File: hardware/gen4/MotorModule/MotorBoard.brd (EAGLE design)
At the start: 32.6 x 58.8 mm, 65 parts, among them IC1 XMEGA16A4A, M1O1 TEST_PT, M1O2 TEST_PT, M1O3 TEST_PT

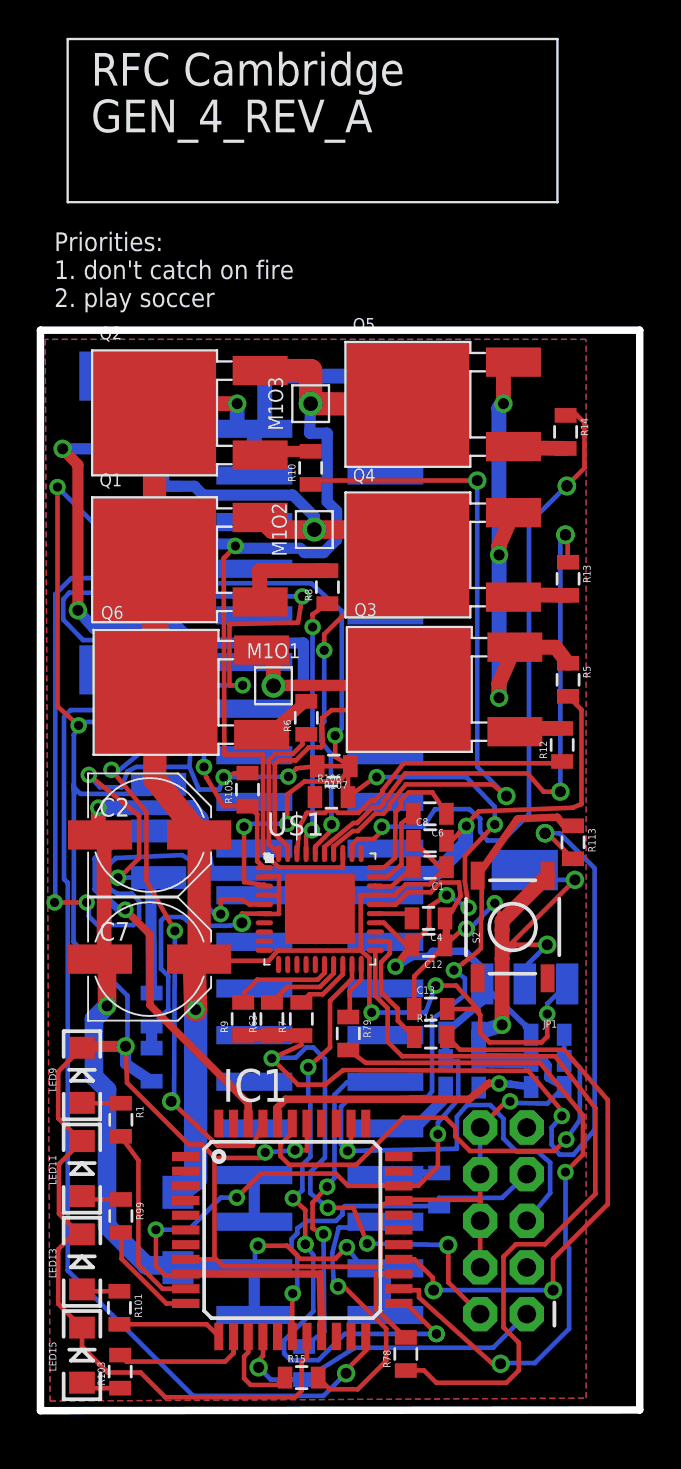
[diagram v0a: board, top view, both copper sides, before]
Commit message: one more airwire to route
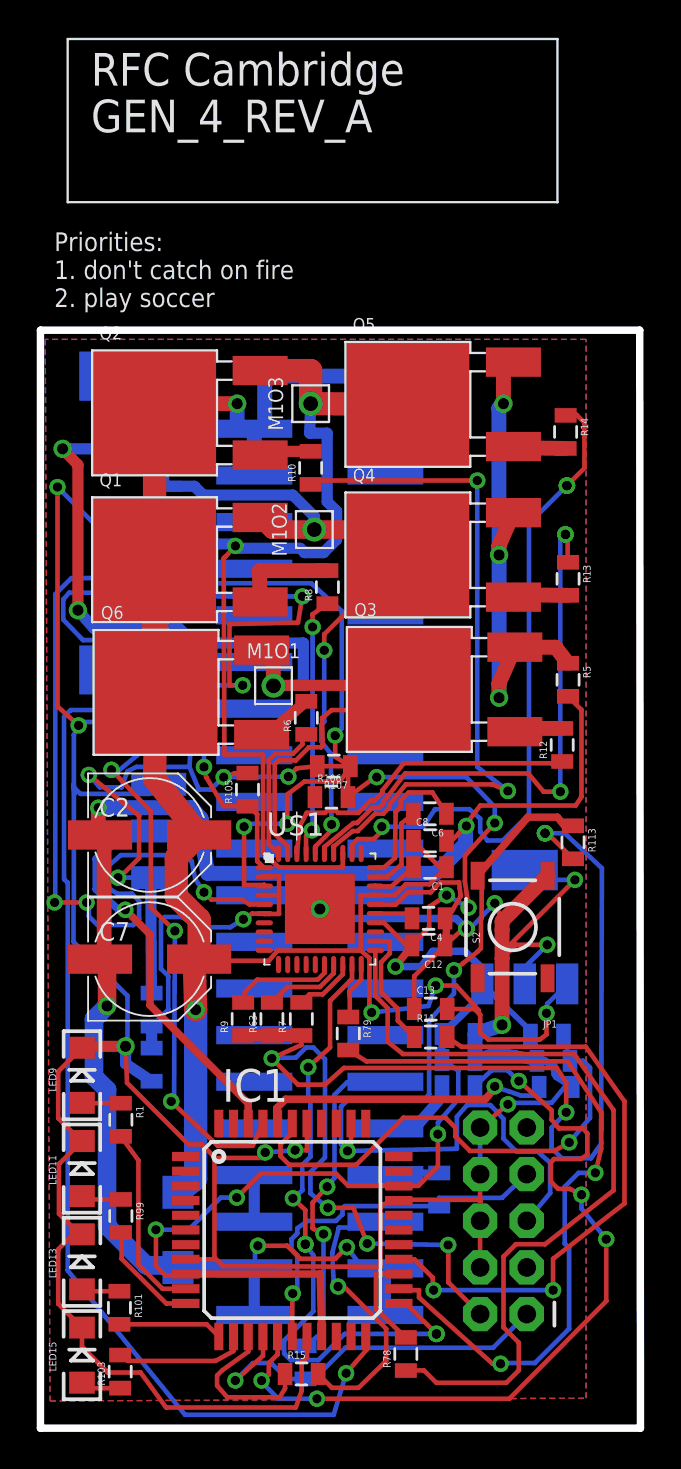
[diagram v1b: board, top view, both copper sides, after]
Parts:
- moved C33 0.44 mm to (27.8, 3.29)
- moved C40 0.32 mm to (27.7, 4.71)
- moved R3 0.21 mm to (22.6, 3.33)
- moved C46 0.21 mm to (22.6, 6.17)
- moved C45 0.20 mm to (22.6, 4.75)
- moved R15 0.20 mm to (14.0, -12.3)
- moved R2 0.09 mm to (14.2, -11.7)
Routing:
- net MISO: track 0.00 -> 44.9 mm, vias 0 -> 5
- net GND: track 206.8 -> 213.9 mm, vias 11 -> 12
- net MOSI: track 17.9 -> 21.7 mm
- net SS_M: track 4.92 -> 8.57 mm
- net VREG: track 72.9 -> 75.7 mm
- net BREN: track 38.3 -> 40.5 mm
- net TSENSE1: track 56.6 -> 58.7 mm
- net ENABLE: track 31.3 -> 33.0 mm
- net N$98: track 42.6 -> 44.3 mm
- net M1H1: track 44.8 -> 43.2 mm
- net RESET: track 49.0 -> 48.1 mm
- net N$8: track 15.2 -> 16.0 mm
- net AVCC: track 26.7 -> 27.4 mm
- net 12V: track 110.9 -> 111.4 mm
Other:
- board size 32.6 x 58.8 mm -> 32.7 x 59.8 mm
